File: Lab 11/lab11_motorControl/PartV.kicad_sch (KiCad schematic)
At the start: 2 parts, among them U4 LM324, U5 NE555D

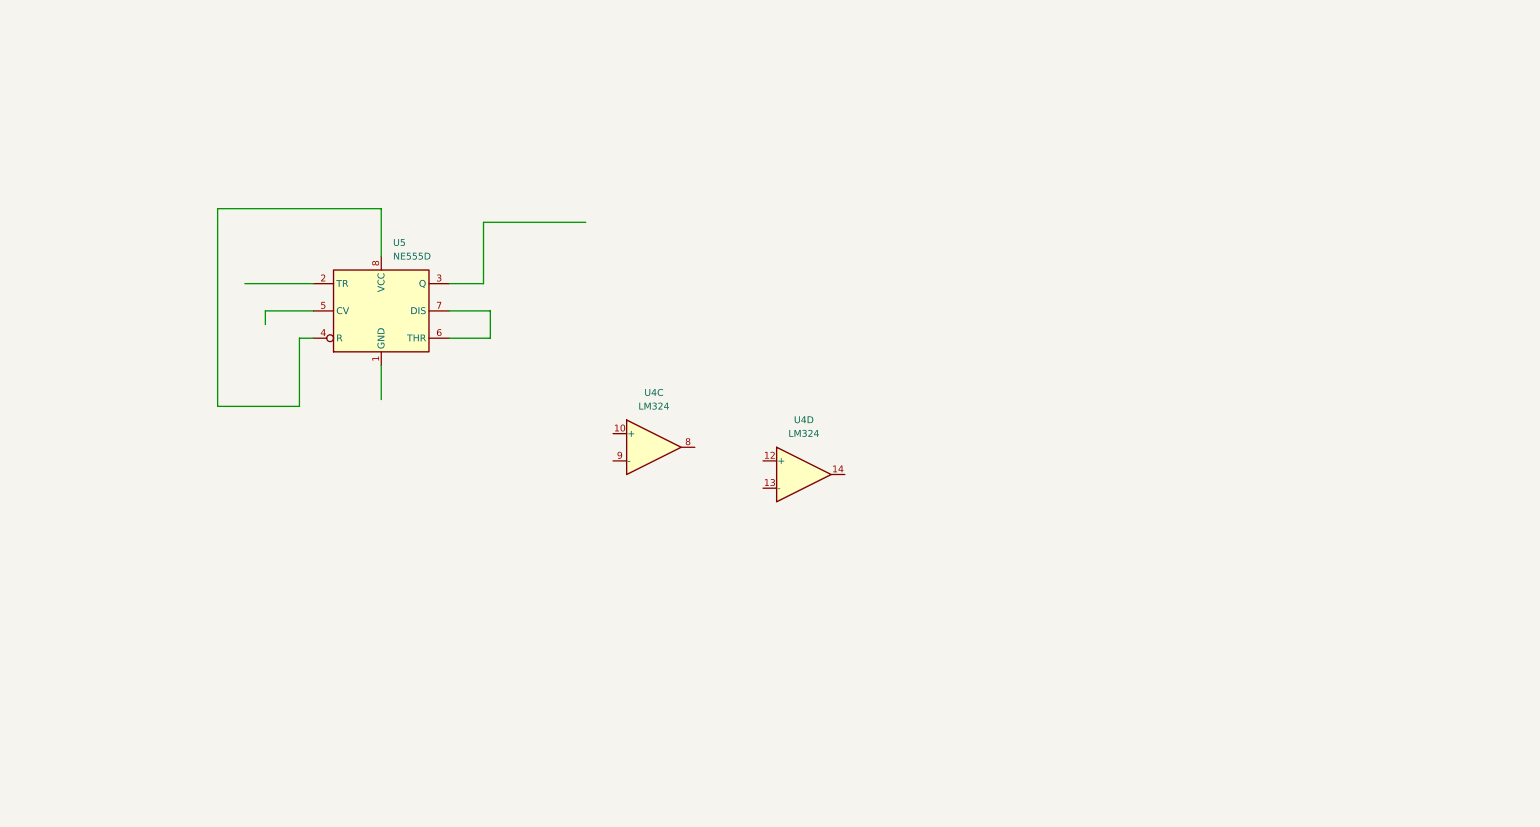
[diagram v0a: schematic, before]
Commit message: Lab 11
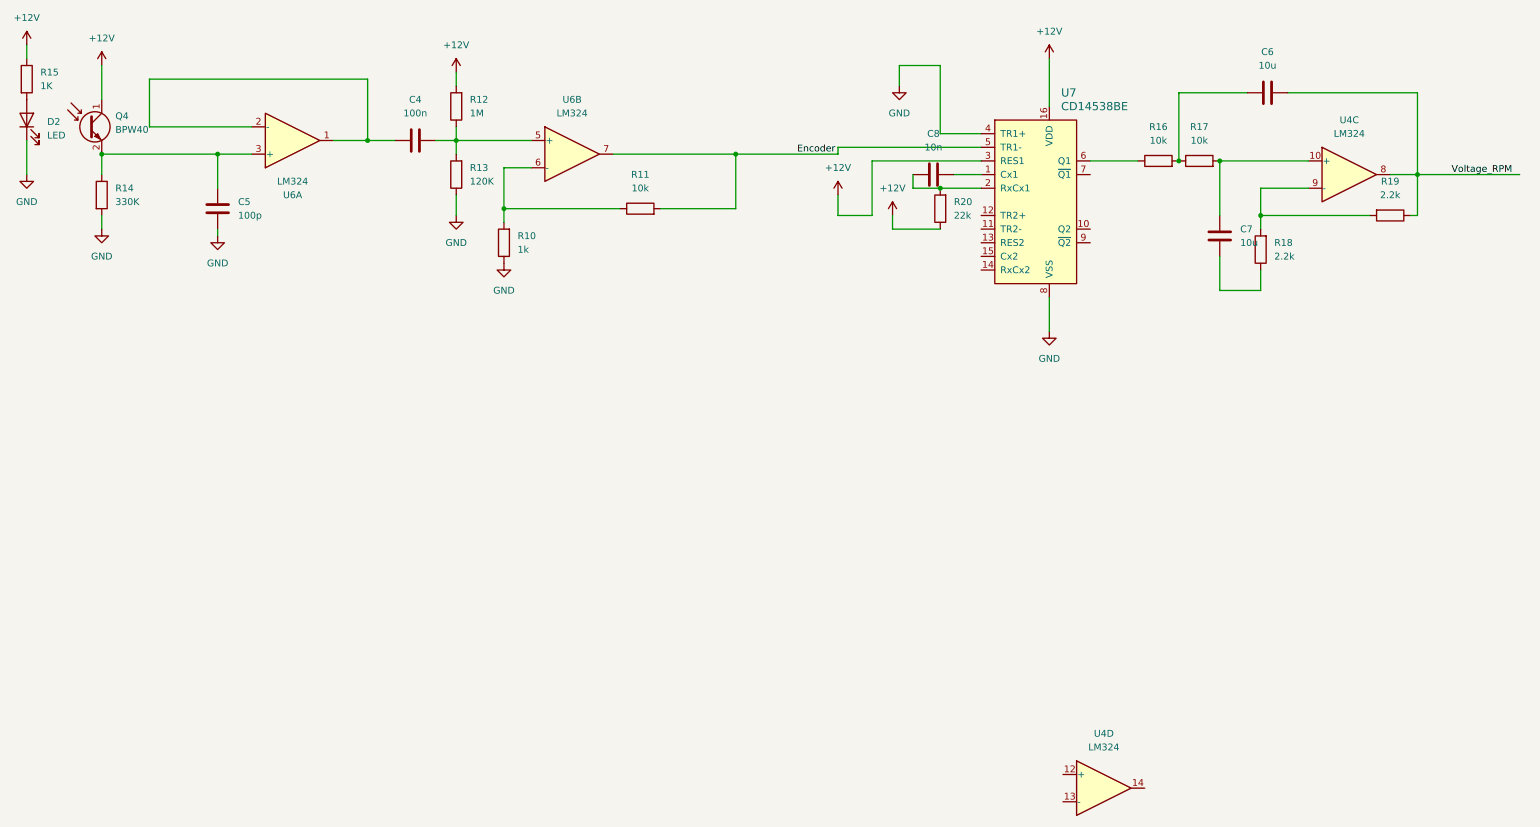
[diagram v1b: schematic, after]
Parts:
- removed U5: NE555D, Package_SO:SOIC-8_3.9x4.9mm_P1.27mm, symbol Timer:NE555D
- added C4: 100n, symbol Device:C
- added C5: 100p, symbol Device:C
- added C6, C7: 10u, symbol Device:C
- added C8: 10n, symbol Device:C
- added D2: LED, symbol Device:LED
- added Q4: BPW40, LED_THT:LED_D5.0mm_Clear, symbol Sensor_Optical:BPW40
- added R10: 1k, symbol Device:R
- added R11, R16, R17: 10k, symbol Device:R
- added R12: 1M, symbol Device:R
- added R13: 120K, symbol Device:R
- added R14: 330K, symbol Device:R
- added R15: 1K, symbol Device:R
- added R18, R19: 2.2k, symbol Device:R
- added R20: 22k, symbol Device:R
- added U6: LM324, symbol Amplifier_Operational:LM324
- added U7: CD14538BE, digikey-footprints:DIP-16_W7.62mm, symbol dk_Logic-Multivibrators:CD14538BE
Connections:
- net at U4.10 (+): now also C7.2, R17.2
- net Voltage_RPM: now reaches U4.8
- net Voltage_RPM: now also C6.2, R19.1
- net at U4.9 (-): now also R18.2, R19.2
- new net: C4.2, R12.1, R13.2, U6.5 (+)
- new net: C7.1, R18.1
- new net: C8.1, R20.2, U7.2 (RxCx1)
- new net: C8.2, U7.1 (Cx1)
- new net: C5.1, Q4.2 (E), R14.1, U6.3 (+)
- new net: C6.1, R16.2, R17.1
- new net: R16.1, U7.6 (Q1)
- new net: R10.2, R11.1, U6.6 (-)
- new net: D2.2 (A), R15.2
- new net: C4.1, U6.1, U6.2 (-)
- new net +12V: Q4.1 (C), R12.2, R15.1, R20.1, U7.16 (VDD), U7.3 (RES1)
- new net Encoder: R11.2, U6.7, U7.5 (TR1-)
- new net GND: C5.2, D2.1 (K), R10.1, R13.1, R14.2, U7.4 (TR1+), U7.8 (VSS)
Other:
- moved on the sheet: U4C, U4D
